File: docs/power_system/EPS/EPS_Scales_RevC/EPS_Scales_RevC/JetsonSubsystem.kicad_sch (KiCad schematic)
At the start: 24 parts, among them U4 INA230

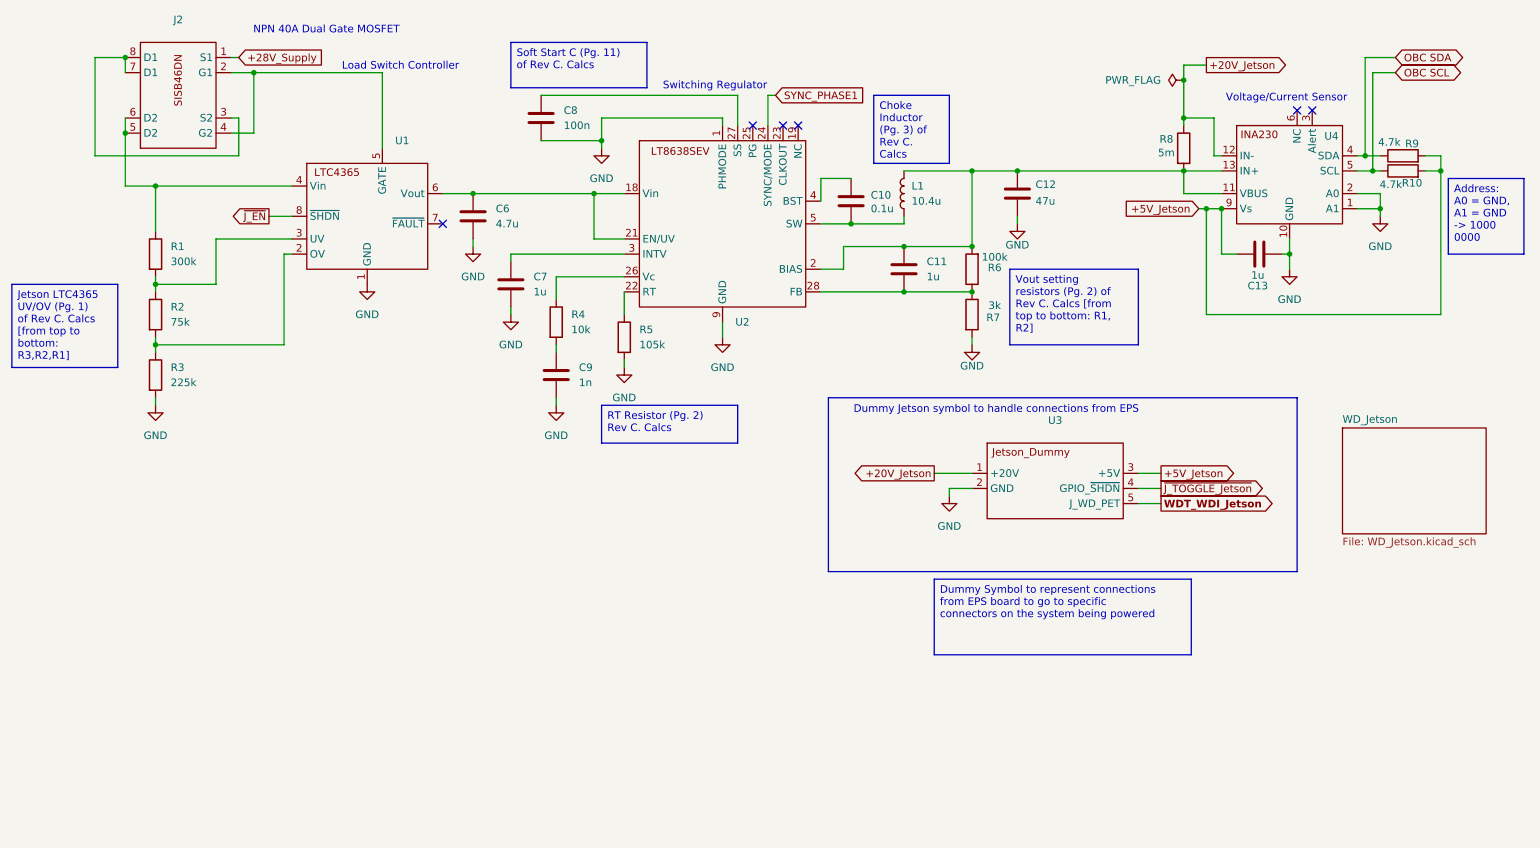
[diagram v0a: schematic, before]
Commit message: Layout Revisions
Organizing components and layering considerations
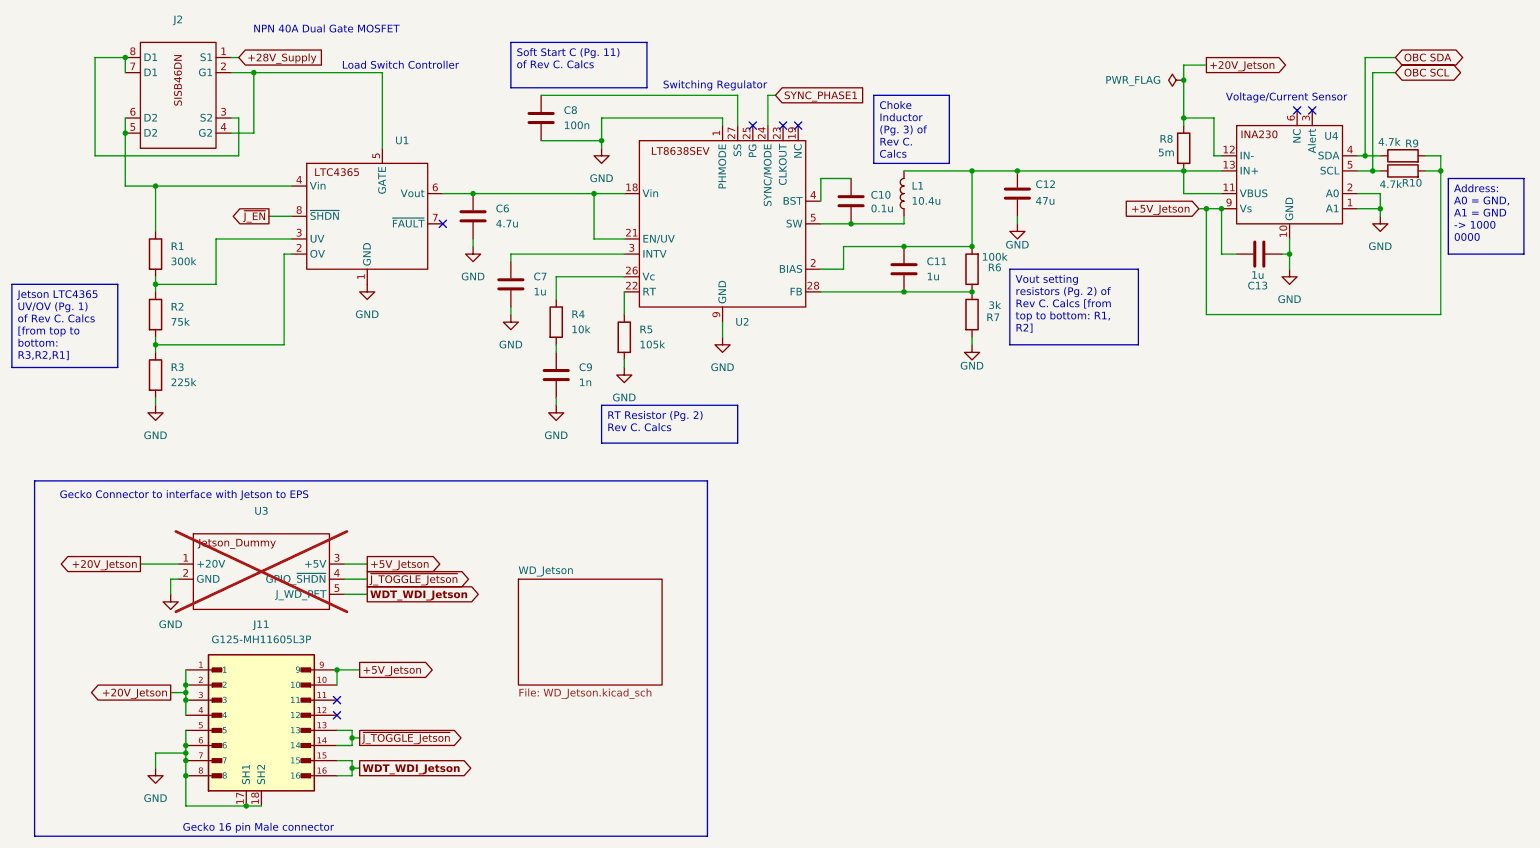
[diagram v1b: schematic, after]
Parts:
- added J11: G125-MH11605L3P, RevC Footprints:HARWIN_G125-MH11605L3P, symbol 16 Pin Gecko Male Connector:G125-MH11605L3P
- U3: now not fitted; now left out of the parts list
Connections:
- net +20V_Jetson: now also J11.1, J11.2, J11.3, J11.4
- net +5V_Jetson: now also J11.10, J11.9
- net GND: now also J11.17 (SH1), J11.18 (SH2), J11.5, J11.6, J11.7, J11.8
- net WDT_WDI_Jetson: now also J11.15, J11.16
- net ~{J_TOGGLE_Jetson}: now also J11.13, J11.14
- no-connect marks 6 -> 8
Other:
- note added: "Gecko 16 pin Male connector"
- note added: "Gecko Connector to interface with Jetson to EPS"
- note removed: "Dummy Jetson symbol to handle connections from EPS"
